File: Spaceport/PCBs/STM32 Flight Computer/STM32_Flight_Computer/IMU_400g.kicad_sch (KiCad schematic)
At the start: 1 part, among them U7 H3LIS331DLTR

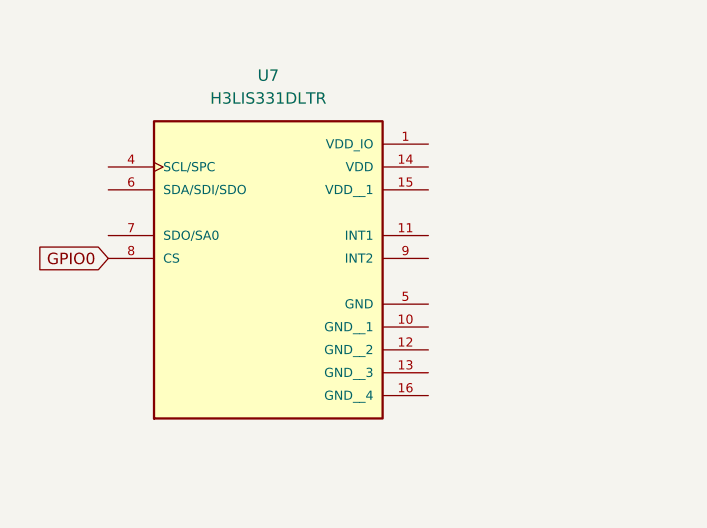
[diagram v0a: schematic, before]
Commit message: Push
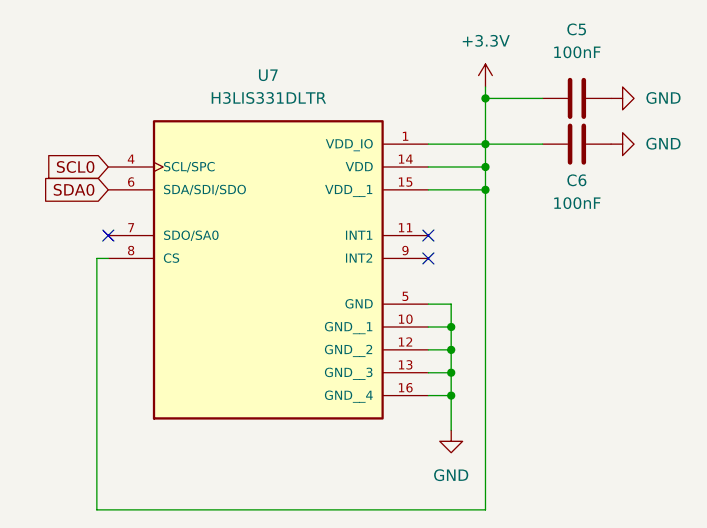
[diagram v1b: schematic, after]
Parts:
- added C5, C6: 100nF, symbol Device:C
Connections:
- net GPIO0 is gone; now on net +3.3V: U7.8 (CS)
- net +3.3V: now reaches U7.1 (VDD_IO)
- net +3.3V: now also U7.14 (VDD), U7.15 (VDD__1), C5.2, C6.1
- net GND: now reaches U7.10 (GND__1)
- net GND: now also U7.12 (GND__2), U7.13 (GND__3), U7.16 (GND__4), U7.5 (GND), C5.1, C6.2
- net SCL0: now reaches U7.4 (SCL/SPC)
- net SDA0: now reaches U7.6 (SDA/SDI/SDO)
- no-connect marks 0 -> 3

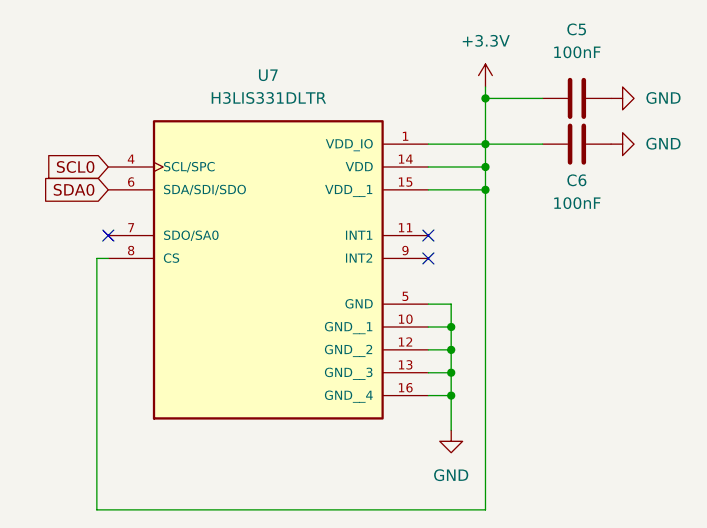
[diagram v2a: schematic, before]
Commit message: Push after Schematic Review 5/5
- Updated STM32 symbol
- Configured I2C busses
- Updated DC caps to 100nF
- TODO add power system things
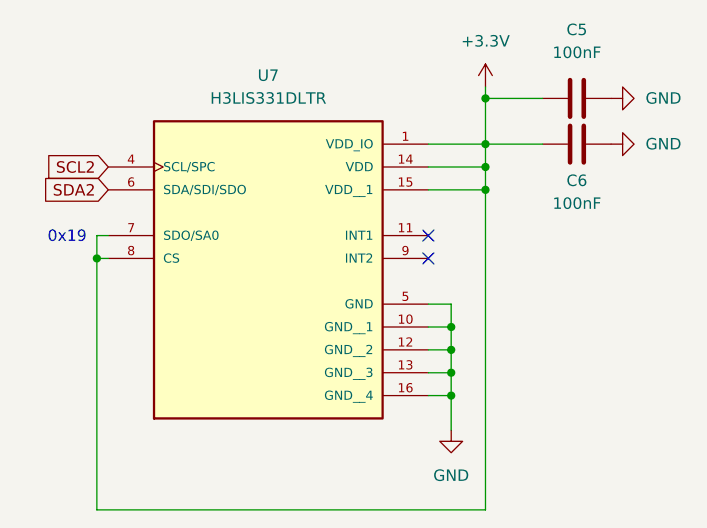
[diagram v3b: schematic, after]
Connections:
- net +3.3V: now also U7.7 (SDO/SA0)
- net SCL0 renamed SCL2
- net SDA0 renamed SDA2
- no-connect marks 3 -> 2
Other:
- note added: "0x19"
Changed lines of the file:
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@@
+		(color 0 0 0 0)
+	)
+	(junction
+		(at 130.81 83.82)
+		(diameter 0)
 		(color 0 0 0 0)
 	)
@@
 	)
 	(no_connect
-		(at 132.08 81.28)
-	)
-	(no_connect
 		(at 167.64 81.28)
 	)
@@
 	(wire
 		(pts
+			(xy 132.08 81.28) (xy 130.81 81.28)
+		)
+		(stroke
+			(width 0)
+			(type default)
+		)
+	)
+	(wire
+		(pts
 			(xy 173.99 73.66) (xy 173.99 76.2)
 		)
@@
 	(wire
 		(pts
+			(xy 130.81 81.28) (xy 130.81 83.82)
+		)
+		(stroke
+			(width 0)
+			(type default)
+		)
+	)
+	(wire
+		(pts
 			(xy 167.64 73.66) (xy 173.99 73.66)
 		)
@@
 		)
 	)
-	(global_label "SDA0"
+	(text "0x19"
+		(exclude_from_sim no)
+		(at 127.508 81.534 0)
+		(effects
+			(font
+				(size 1.27 1.27)
+			)
+		)
+	)
+	(global_label "SDA2"
 		(shape input)
 		(at 132.08 76.2 180)
@@
 		)
 	)
-	(global_label "SCL0"
+	(global_label "SCL2"
 		(shape input)
 		(at 132.08 73.66 180)
